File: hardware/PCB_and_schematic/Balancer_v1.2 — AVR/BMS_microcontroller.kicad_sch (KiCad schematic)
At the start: 60 parts, among them J10 RS485, J2 VOLTAGE_3WIRE, J8 ICP, J9 RS485, Q17 BC817, Q19 BC817, Q20 BC817, Q21 BC817, Q22 BC817, U4 TL432DBZ, U6 ST485, U7 INA226, U8 AVR64DD28

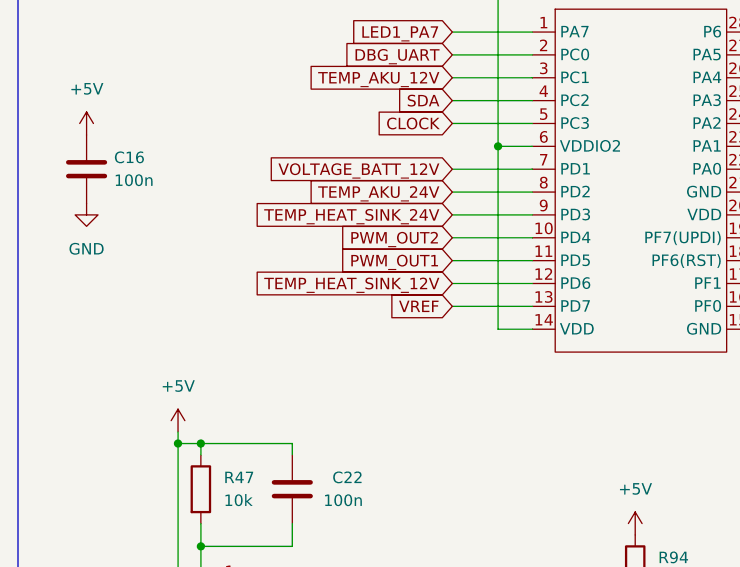
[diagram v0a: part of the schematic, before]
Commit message: Add PWM code
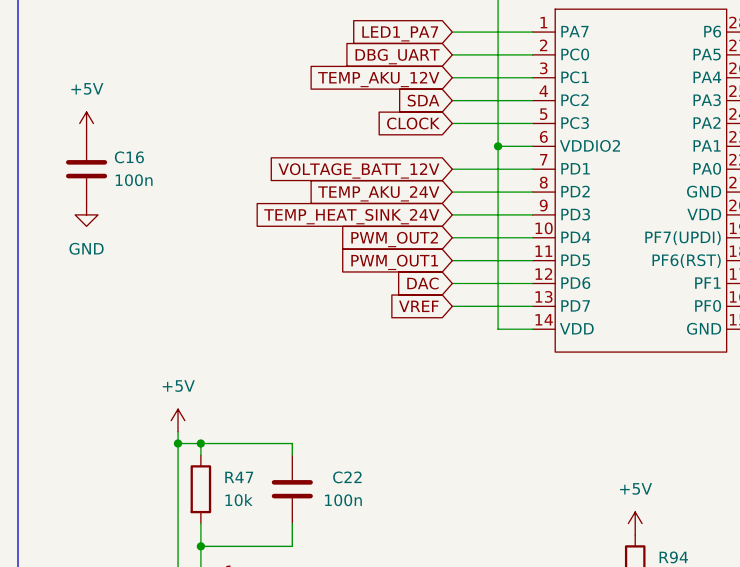
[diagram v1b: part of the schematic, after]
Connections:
- net TEMP_HEAT_SINK_12V renamed DAC
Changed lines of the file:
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@@
 		)
 	)
-	(global_label "TEMP_HEAT_SINK_12V"
+	(global_label "DAC"
 		(shape input)
 		(at 72.39 86.36 180)
@@
 		)
 		(property "Intersheetrefs" "${INTERSHEET_REFS}"
-			(at 49.2059 86.36 0)
+			(at 65.7762 86.36 0)
 			(effects
 				(font

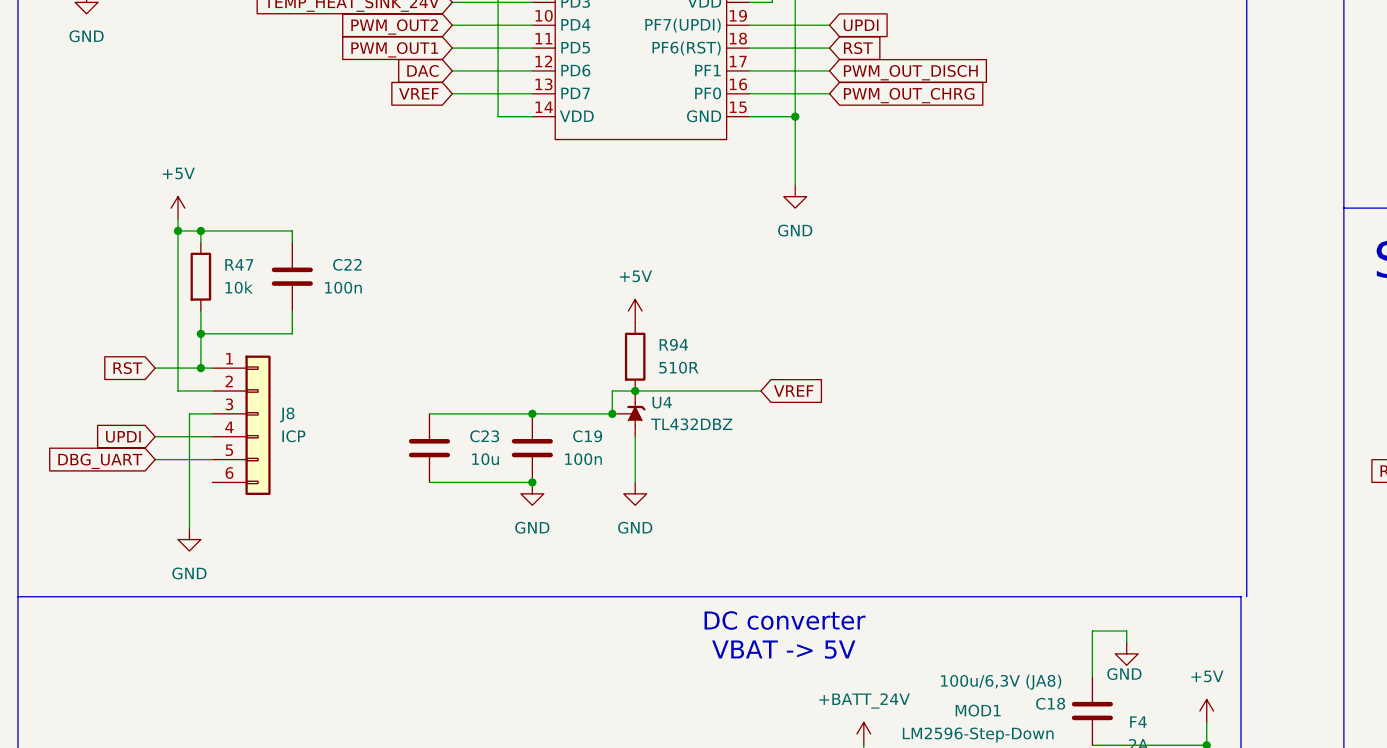
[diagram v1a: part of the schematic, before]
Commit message: New schematic BMS
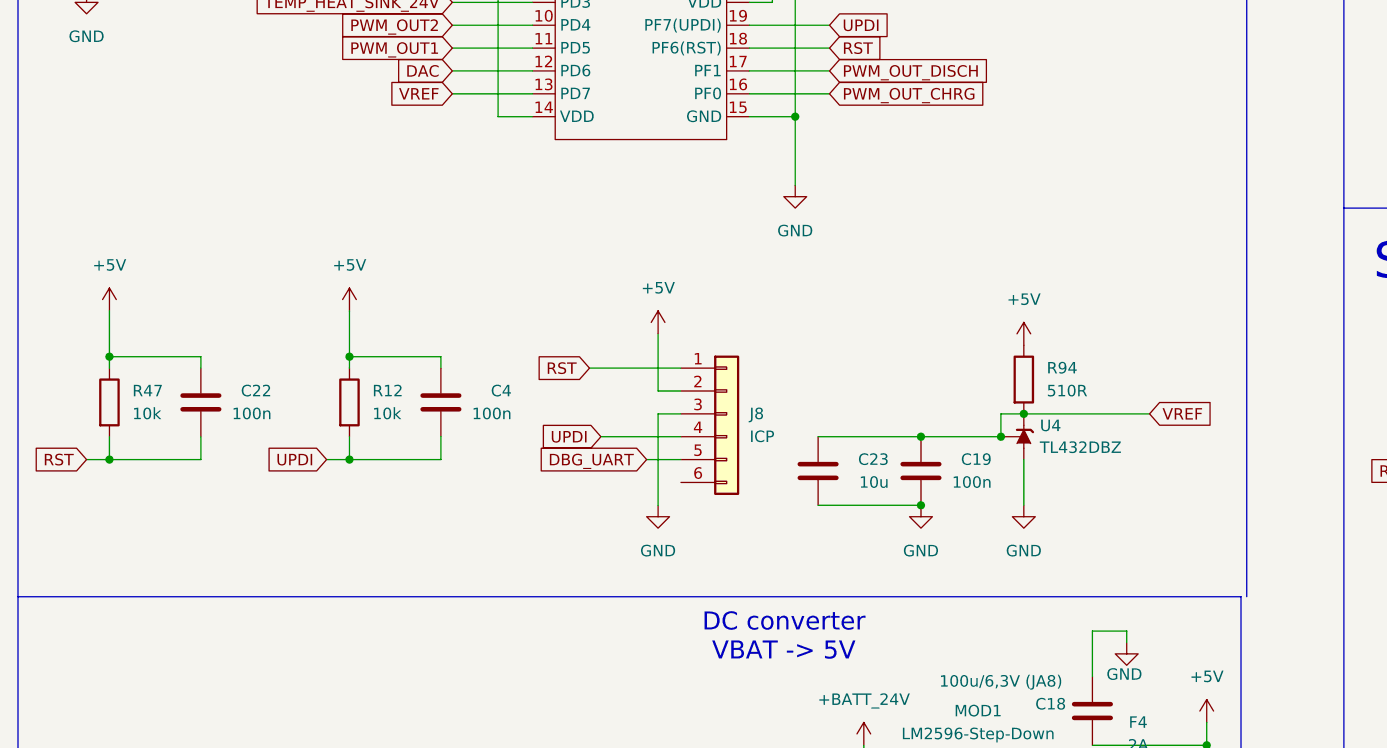
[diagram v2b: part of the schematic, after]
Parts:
- added C4: 100n, Capacitor_SMD:C_0805_2012Metric_Pad1.18x1.45mm_HandSolder, symbol Device:C
- added R12: 10k, Resistor_SMD:R_0805_2012Metric_Pad1.20x1.40mm_HandSolder, symbol Device:R
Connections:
- net +5V: now also C4.1, R12.1
- net UPDI: now also C4.2, R12.2
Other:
- moved on the sheet: C19, C22, C23, J8, R47, R94, U4
